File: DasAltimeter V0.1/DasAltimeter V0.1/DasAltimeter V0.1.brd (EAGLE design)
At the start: 39.6 x 21.8 mm, 57 parts, among them IC1 BMI055, U1 ATSAMD21G-A, U2 3.3V/150mA, U3 MS5803-14BA, U4 ADXL193, X1 22-23-2041, X2 22-23-2041, Y1 32.768kHz

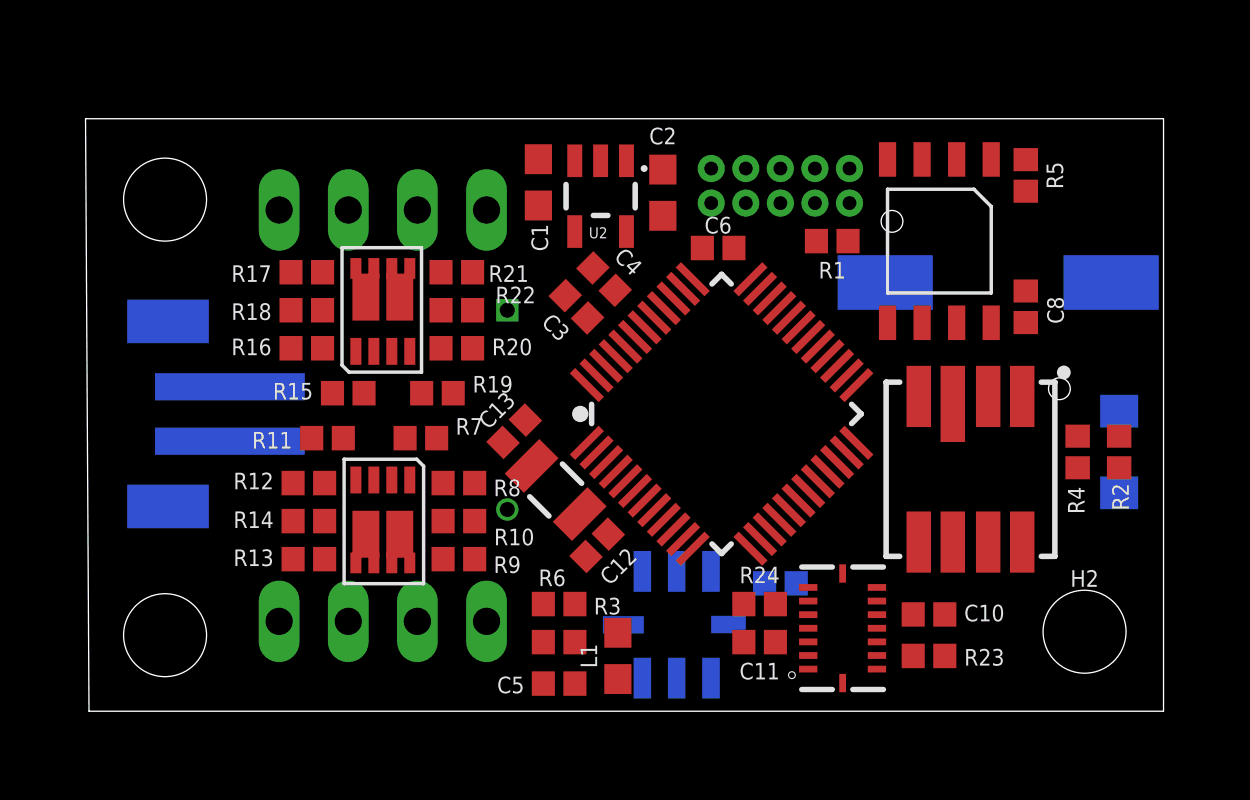
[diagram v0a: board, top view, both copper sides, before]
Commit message: V0.1 board
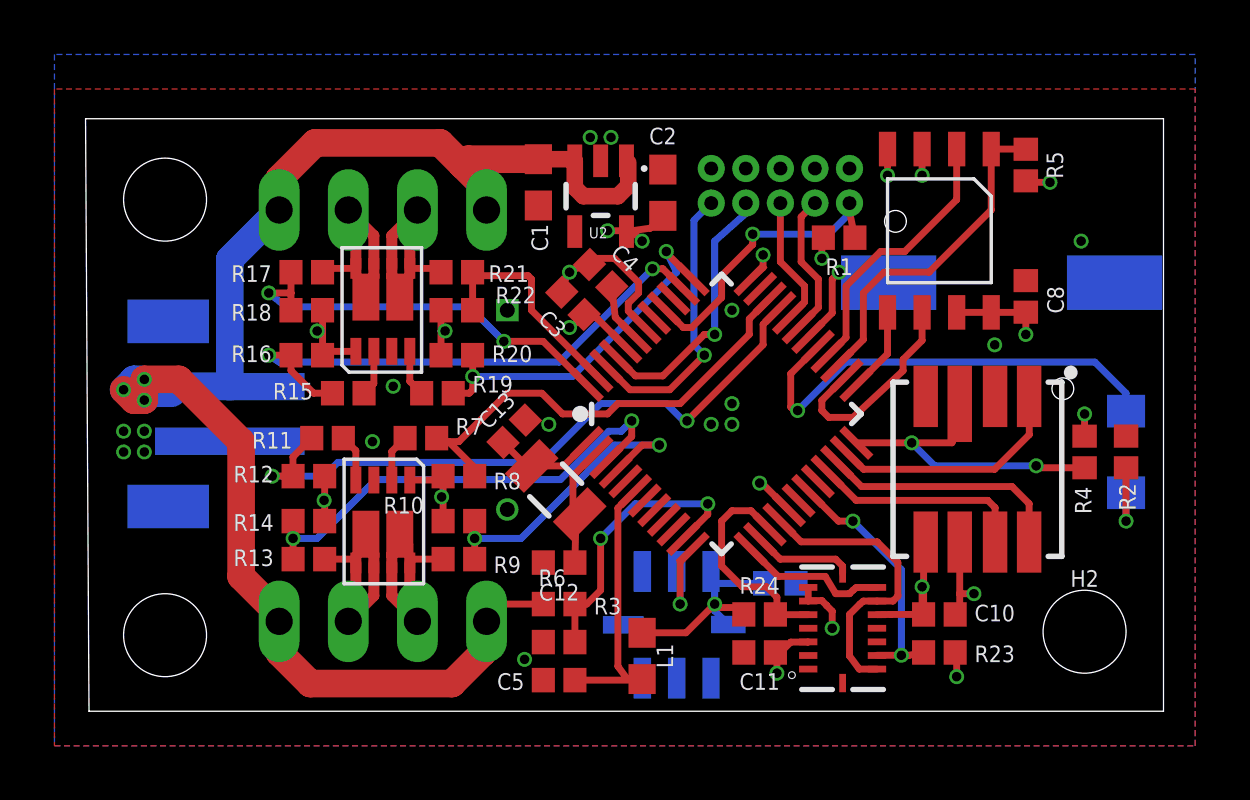
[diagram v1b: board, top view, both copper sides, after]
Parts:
- removed C6: 0.1uF, SparkFun-Capacitors:0402
- moved C12 1.53 mm to (17.3, 5.46), turned to 0 degrees
- moved L1 0.89 mm to (20.3, 2.03)
- moved R23 0.40 mm to (31.2, 2.16)
- moved C10 0.38 mm to (31.2, 3.56)
- moved C11 0.38 mm to (24.6, 2.16)
- moved C8 0.38 mm to (34.4, 15.2)
- moved MEM 0.38 mm to (30.6, 17.7)
- moved R5 0.38 mm to (34.4, 20.1)
- moved R24 0.38 mm to (24.6, 3.56)
- moved R1 0.28 mm to (27.6, 17.4)
- moved D2 0.25 mm to (38.1, 9.53)
- moved R2 0.25 mm to (38.1, 9.53)
- moved U3 0.25 mm to (32.6, 8.89)
- moved R16 0.25 mm to (8.00, 13.1)
- moved R20 0.25 mm to (13.5, 13.1)
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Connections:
- removed net N$11: U1.33
- removed net N$14: U1.34
- removed net RESET: R1.1, U1.40
- new net RX: JP1.6, U1.32
- new net TX: JP1.8, U1.31
- net !RESET: now also R1.1, U1.40
- net 3.3V: no longer C6.1
- net BUZZER: now also U1.30; no longer U1.31
- net CS_ACCEL: now also U1.19; no longer U1.15
- net CS_BARO: now also U1.24; no longer U1.23
- net CS_GYRO: now also U1.15; no longer U1.19
- net FIRE_A: now also U1.38
- net FIRE_B: now also U1.37
- net FIRE_C: now also U1.34
- net FIRE_D: now also U1.33
- net GND: now also U1.18, U1.35, U1.42, U1.5; no longer C6.2
- net LED: now also U1.29
- net SENSE_A: now also U1.48; no longer U1.47
- net SENSE_B: now also U1.47; no longer U1.48
- net SPI2_MISO: now also U1.22; no longer U1.24
- net SPI2_SCK: now also U1.23; no longer U1.22
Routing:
- net VCC: track 0.00 -> 58.2 mm, vias 0 -> 3
- net 3.3V: track 0.00 -> 32.2 mm, vias 0 -> 14
- net FIRE_D: track 0.00 -> 24.6 mm, vias 0 -> 2
- net GND: track 0.00 -> 22.3 mm, vias 0 -> 24
- net FIRE_A: track 0.00 -> 20.3 mm, vias 0 -> 2
- net SENSE_D: track 0.00 -> 17.5 mm, vias 0 -> 2
- net FIRE_C: track 0.00 -> 17.4 mm
- net LED: track 0.00 -> 16.9 mm, vias 0 -> 1
- net SENSE_A: track 0.00 -> 15.3 mm, vias 0 -> 2
- net FIRE_B: track 0.00 -> 13.9 mm, vias 0 -> 2
- net CS_MEM: track 0.00 -> 12.5 mm
- net CS_BARO: track 0.00 -> 11.7 mm, vias 0 -> 2
- net SENSE_C: track 0.00 -> 11.6 mm, vias 0 -> 2
- net !RESET: track 0.00 -> 11.2 mm, vias 0 -> 1
- net SPI0_MISO: track 0.00 -> 11.1 mm
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- added copper zone on layer 15, net 3.3V
- added copper zone on layer 1, net GND
- added copper zone on layer 16, net GND
- added copper zone on layer 2, net GND
